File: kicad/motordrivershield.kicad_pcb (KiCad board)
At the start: 2 copper layers, 100 x 60 mm, 155 parts, among them CN1 ARDUINO_MKR, CN2 QWIIC, CN3 ARDUINO_NANO_33, P1 CONN_01X03, P2 CONN_01X03, P5 WR-TBL_691313710002, P6 WR-TBL_691313710002, P7 CONN_01X02, P8 WR-TBL_691313710002, U1 PCA9685_TSSOP28, U10 IFX007T, U11 74xx32, U2 ADS1015, U3 LT1117, U4 TPS54335A, U5 LM358, U6 IFX007T, U7 IFX007T, U8 LM358, U9 IFX007T

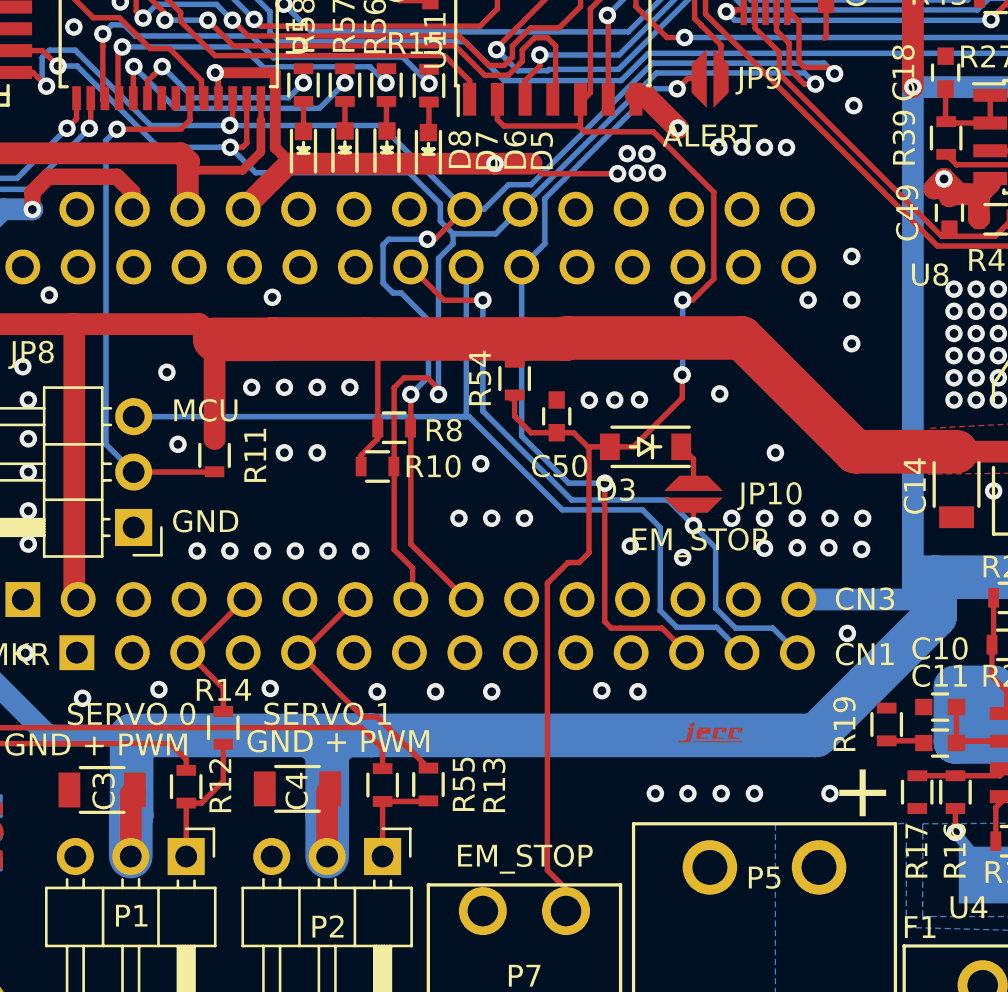
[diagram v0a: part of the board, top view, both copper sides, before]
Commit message: servos angepasst
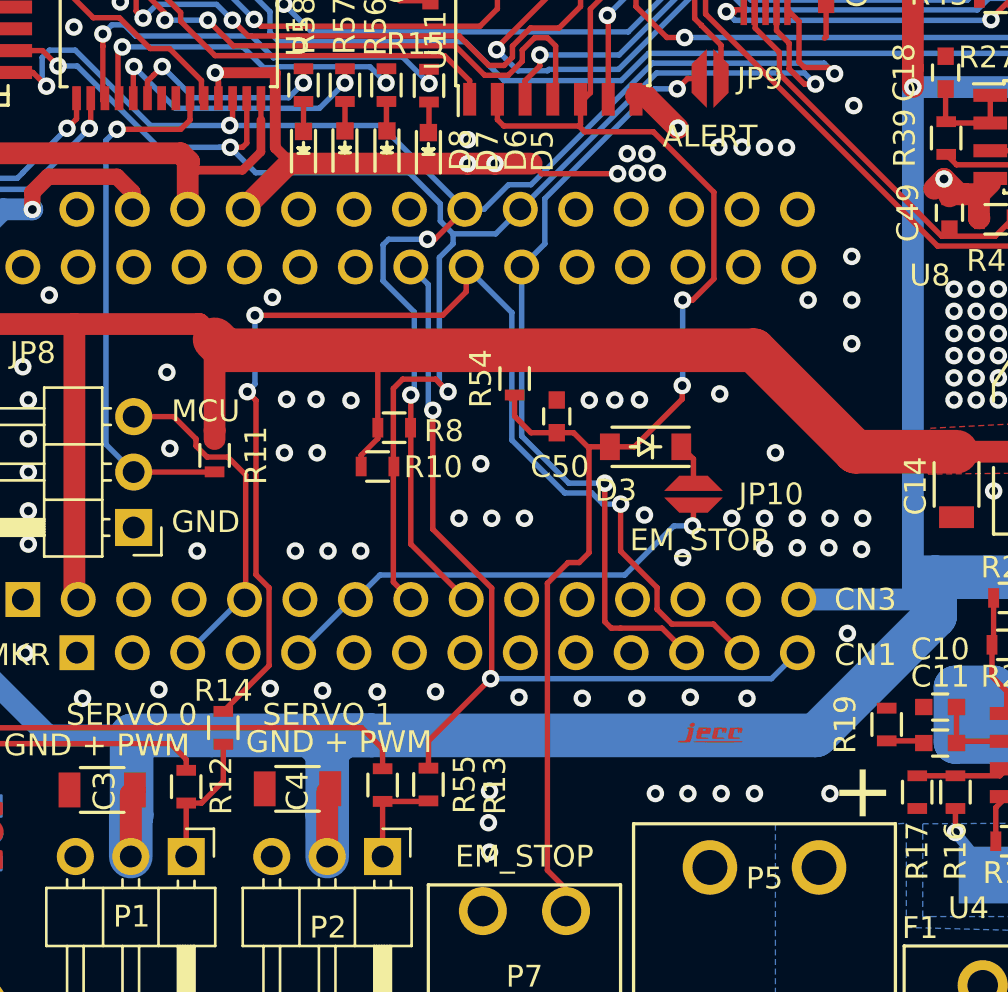
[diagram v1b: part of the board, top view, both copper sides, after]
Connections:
- CN1 pad 13: /~OE_MCU -> /SERVO0_MCU
- CN1 pad 14: /EM_MCU -> /SERVO1_MCU
- CN1 pad 3: /SERVO0_MCU -> /~OE_MCU
- CN1 pad 5: /SERVO1_MCU -> /EM_MCU
- CN3 pad 22: /~OE_MCU -> /SERVO0_MCU
- CN3 pad 23: /EM_MCU -> /SERVO1_MCU
- CN3 pad 5: /SERVO0_MCU -> /~OE_MCU
- CN3 pad 7: /SERVO1_MCU -> /EM_MCU
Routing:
- net /SERVO0_MCU: track 6.98 -> 56.1 mm, vias 0 -> 3
- net /SERVO1_MCU: track 11.8 -> 40.3 mm, vias 0 -> 2
- net /~OE_MCU: track 43.0 -> 15.8 mm
- net /EM_MCU: track 30.6 -> 21.4 mm, vias 2 -> 1
- net /SCL: track 74.5 -> 73.7 mm
- net GND: vias 223 -> 228

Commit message: blöder servo
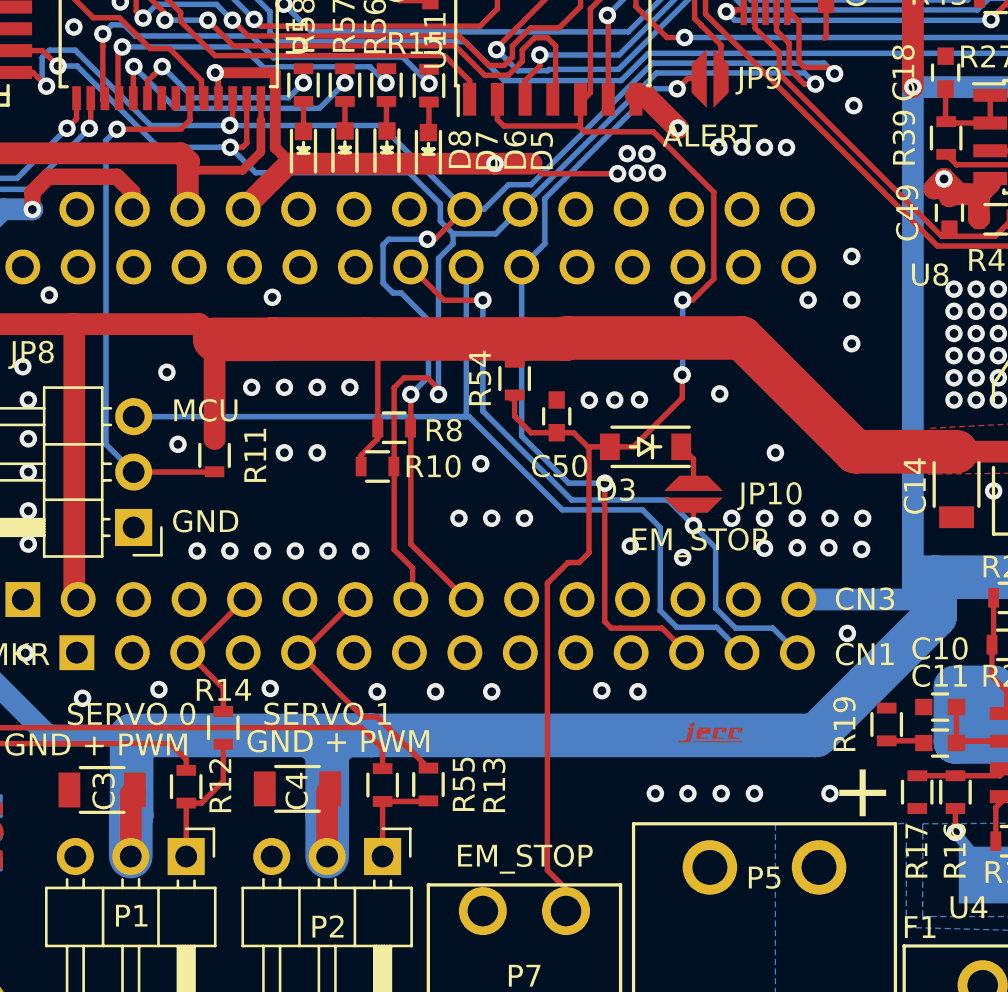
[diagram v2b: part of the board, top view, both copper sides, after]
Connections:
- CN1 pad 13: /SERVO0_MCU -> /~OE_MCU
- CN1 pad 14: /SERVO1_MCU -> /EM_MCU
- CN1 pad 3: /~OE_MCU -> /SERVO0_MCU
- CN1 pad 5: /EM_MCU -> /SERVO1_MCU
- CN3 pad 22: /SERVO0_MCU -> /~OE_MCU
- CN3 pad 23: /SERVO1_MCU -> /EM_MCU
- CN3 pad 5: /~OE_MCU -> /SERVO0_MCU
- CN3 pad 7: /EM_MCU -> /SERVO1_MCU
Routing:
- net /SERVO0_MCU: track 56.1 -> 6.98 mm, vias 3 -> 0
- net /SERVO1_MCU: track 40.3 -> 11.8 mm, vias 2 -> 0
- net /~OE_MCU: track 15.8 -> 43.0 mm
- net /EM_MCU: track 21.4 -> 30.6 mm, vias 1 -> 2
- net /SCL: track 73.7 -> 74.5 mm
- net GND: vias 228 -> 223
